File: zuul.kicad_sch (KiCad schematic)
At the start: 8 parts, among them IC1 DRV8251DDAR, J1 Raspberry_Pi_2_3, J2 MOTOR_OUTPUT, J5 Conn_01x06_Male

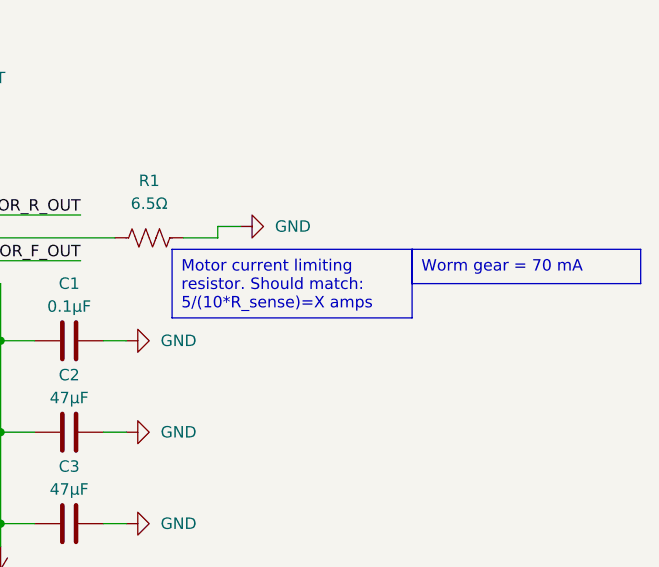
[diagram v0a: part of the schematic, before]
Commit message: ummm
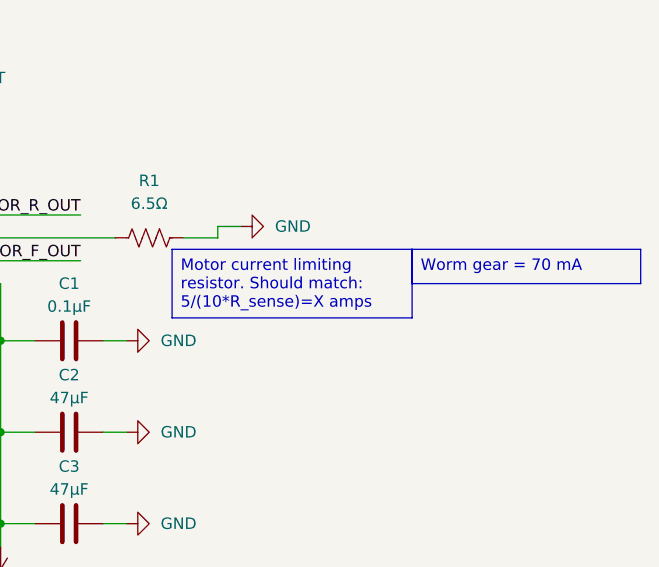
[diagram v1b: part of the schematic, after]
